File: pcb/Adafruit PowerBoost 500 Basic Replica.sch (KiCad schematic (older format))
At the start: 24 parts, among them CN1 USBA, J1 HEADER, J2 PWR OUT CONN, Q1 MMUN2133LT1G, U1 TPS61090RSAR

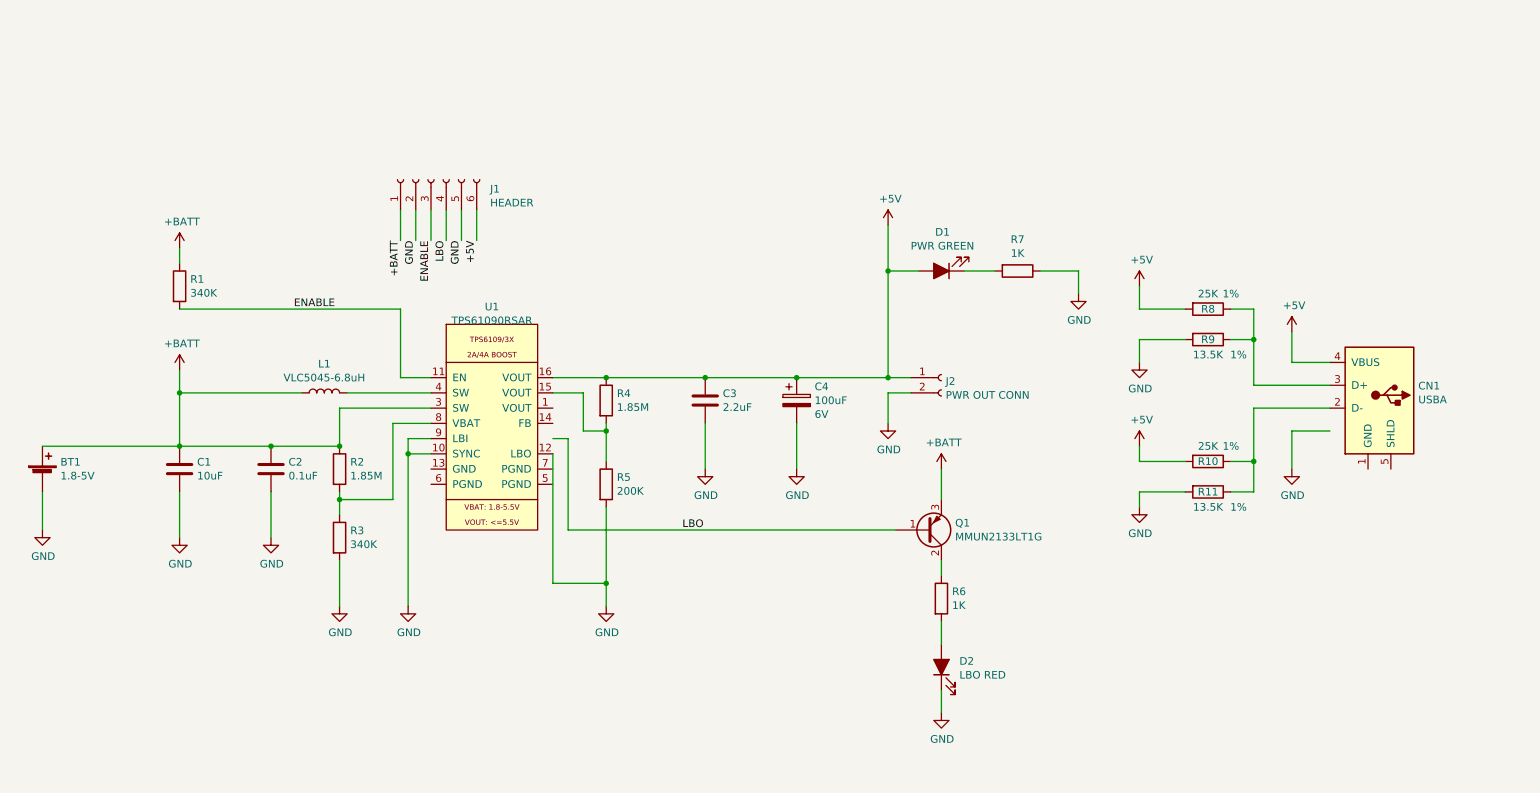
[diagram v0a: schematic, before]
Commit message: Agregada la propuesta
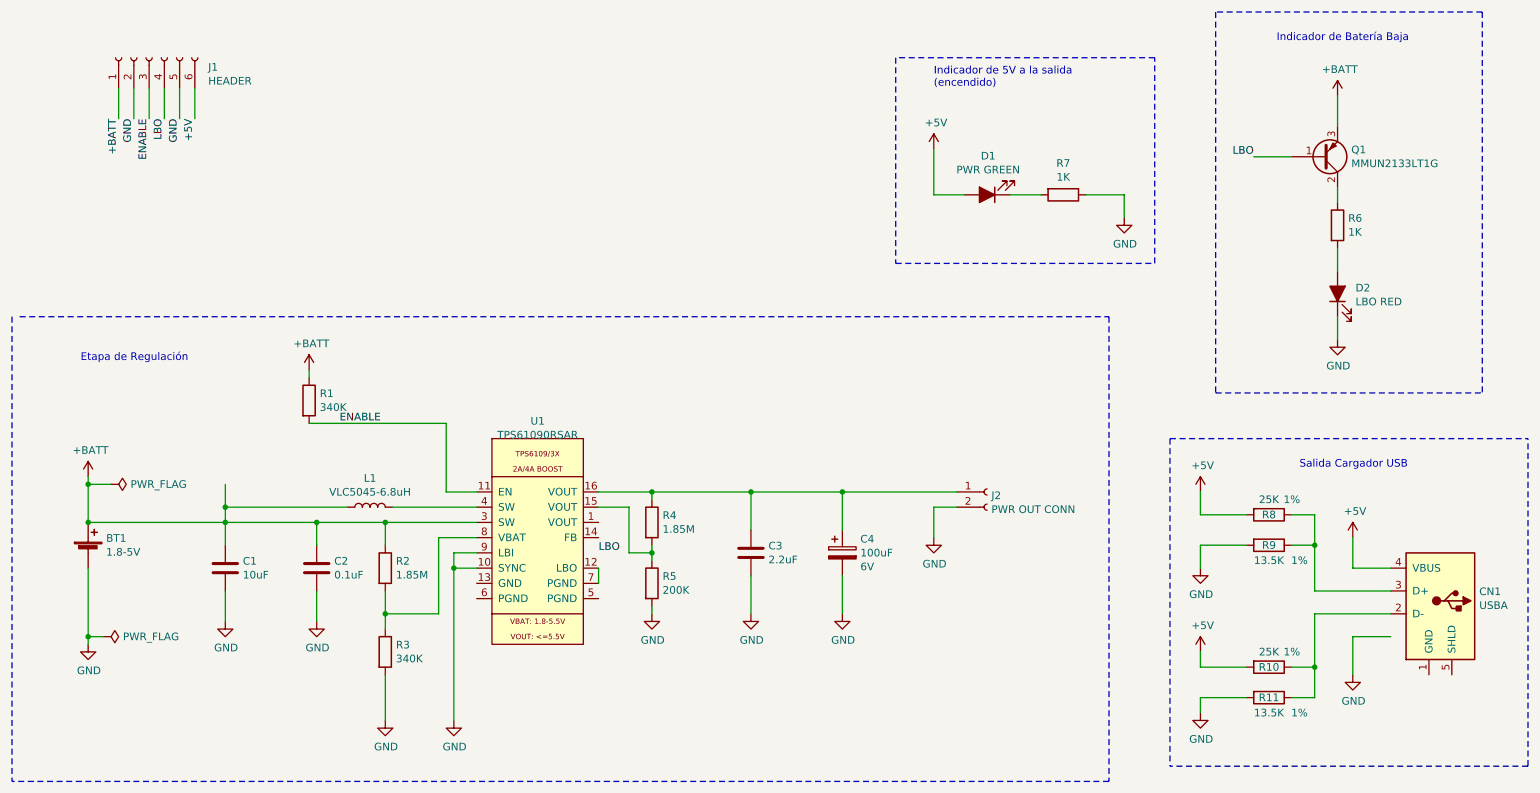
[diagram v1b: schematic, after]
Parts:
- BT1: footprint (none) -> Connector_JST:JST_EH_S2B-EH_1x02_P2.50mm_Horizontal
- C1, C2, C3: footprint (none) -> Capacitor_SMD:C_0805_2012Metric
- C4: footprint (none) -> Capacitor_SMD:C_1206_3216Metric
- CN1: footprint (none) -> Connector_USB:USB_A_CONNFLY_DS1095-WNR0
- D1, D2: footprint (none) -> LED_SMD:LED_0805_2012Metric
- J1: footprint (none) -> Connector_PinHeader_1.00mm:PinHeader_1x06_P1.00mm_Vertical
- J2: footprint (none) -> Connector_PinHeader_1.00mm:PinHeader_1x02_P1.00mm_Vertical
- L1: footprint (none) -> Inductor_SMD:L_TDK_VLP8040
- Q1: footprint (none) -> Package_TO_SOT_SMD:SOT-23
- R1, R10, R11, R2, R3, R4, R5, R6, R7, R8, R9: footprint (none) -> Resistor_SMD:R_0805_2012Metric
- U1: footprint (none) -> Package_DFN_QFN:QFN-16-1EP_4x4mm_P0.65mm_EP2.1x2.1mm
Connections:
- net +5V: no longer C3.1, C4.1, J2.1 (Pin_1), R4.1, U1.16 (VOUT)
- net GND: no longer U1.12 (LBO)
- net at U1.7 (PGND): now also U1.12 (LBO)
- new net: C3.1, C4.1, J2.1 (Pin_1), R4.1, U1.16 (VOUT)
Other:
- note added: "Etapa de Regulación"
- note added: "Indicador de 5V a la salida\n(encendido)"
- note added: "Indicador de Batería Baja"
- note added: "Salida Cargador USB"
- moved on the sheet: BT1, C1, C2, C3, C4, CN1, D1, D2, J1, J2, L1, Q1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
